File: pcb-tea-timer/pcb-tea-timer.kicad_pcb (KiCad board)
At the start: 2 copper layers, 57.2 x 69.8 mm, 4 parts, among them J1 Conn_01x07_Female, Q1 2N7002

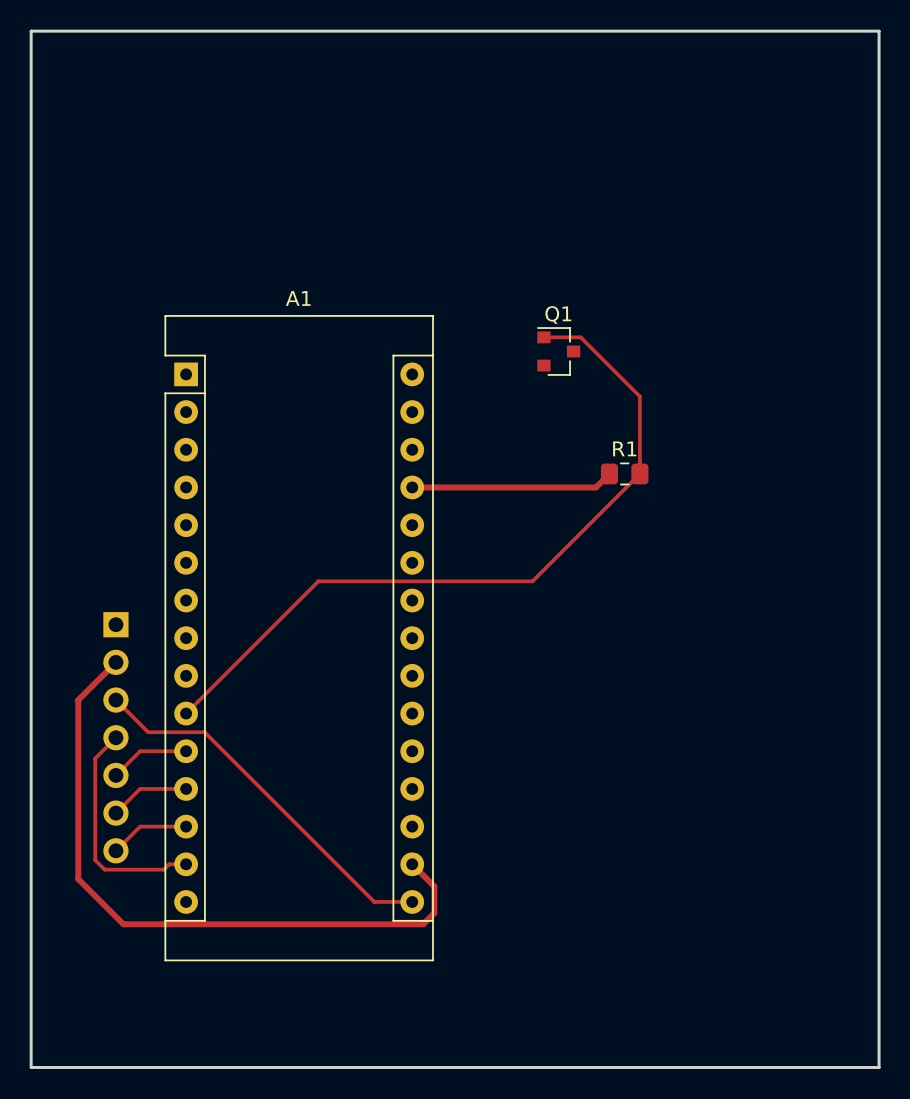
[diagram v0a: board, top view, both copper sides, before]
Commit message: Tea timer PCB finished.
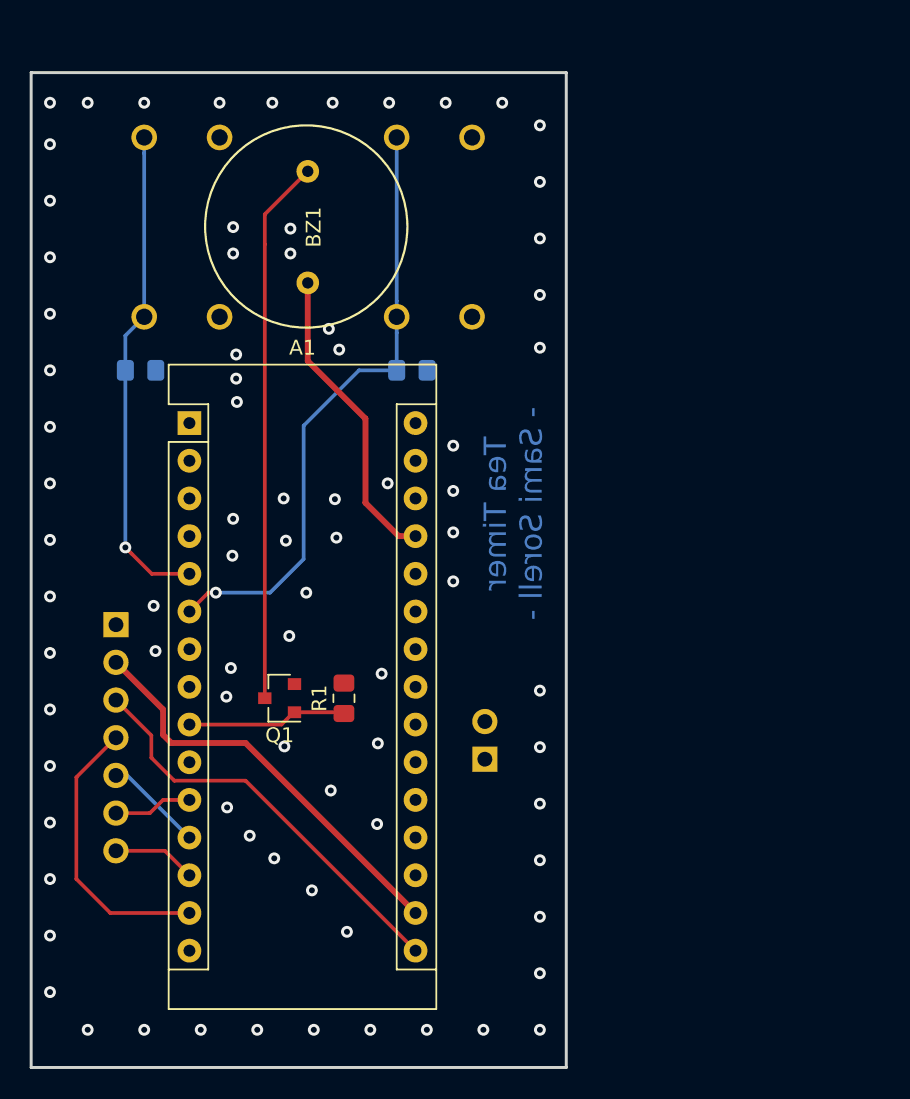
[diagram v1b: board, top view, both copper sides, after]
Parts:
- added BZ1: Buzzer, SS_Connectors:Round Piezo 1, F.Cu at (139.2, 70.4)
- added C1: 1nF, Capacitor_SMD:C_0805_2012Metric_Pad1.15x1.40mm_HandSolder, B.Cu at (128.0, 80.0)
- added C2: 1nF, Capacitor_SMD:C_0805_2012Metric_Pad1.15x1.40mm_HandSolder, B.Cu at (146.3, 80.0)
- added J2: Conn_01x02_Female, Connector_PinHeader_2.54mm:PinHeader_1x02_P2.54mm_Vertical, B.Cu at (151.2, 106.2)
- added SW1: SW_Push_Dual, SS_Connectors:Push Button 12x12mm, B.Cu at (130.8, 70.4)
- added SW2: SW_Push_Dual, SS_Connectors:Push Button 12x12mm, B.Cu at (147.8, 70.4)
- moved Q1 30.0 mm to (137.4, 102.1), turned to 180 degrees
- moved R1 24.2 mm to (141.7, 102.1), turned to 90 degrees
- moved A1 3.29 mm to (131.3, 83.6)
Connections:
- J1 pad 5: Net-(A1-Pad11) -> Net-(A1-Pad12)
- J1 pad 6: Net-(A1-Pad12) -> Net-(A1-Pad11)
- Q1 pad 1: Net-(A1-Pad10) -> Net-(A1-Pad9)
- R1 pad 1: +5V -> Net-(A1-Pad9)
- R1 pad 2: Net-(A1-Pad10) -> GND
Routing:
- net Net-(A1-Pad10): track 50.6 -> 0.00 mm
- net Net-(A1-Pad6): track 0.00 -> 41.7 mm, vias 0 -> 1
- net Net-(BZ1-Pad2): track 0.00 -> 36.7 mm
- net Net-(A1-Pad5): track 0.00 -> 33.2 mm, vias 0 -> 1
- net +3V3: track 45.1 -> 28.2 mm
- net Net-(A1-Pad9): track 0.00 -> 10.8 mm
- net +5V: track 13.7 -> 20.8 mm
- net Net-(A1-Pad14): track 15.4 -> 19.2 mm
- net Net-(A1-Pad16): track 25.6 -> 28.1 mm
- net Net-(A1-Pad12): track 5.41 -> 6.69 mm
- net GND: vias 0 -> 81
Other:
- board size 57.2 x 69.8 mm -> 36.1 x 67.1 mm
- board text added: "CS"
- board text added: "DC"
- board text added: "GND"
- board text added: "RES"
- board text added: "SCL"
- board text added: "SDA"
- board text added: "Tea Timer - Sami Sorell -"
- board text added: "VCC"
